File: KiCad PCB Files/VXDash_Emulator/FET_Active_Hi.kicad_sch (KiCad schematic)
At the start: 11 parts, among them J8 Manual backup, Q24 2N7002

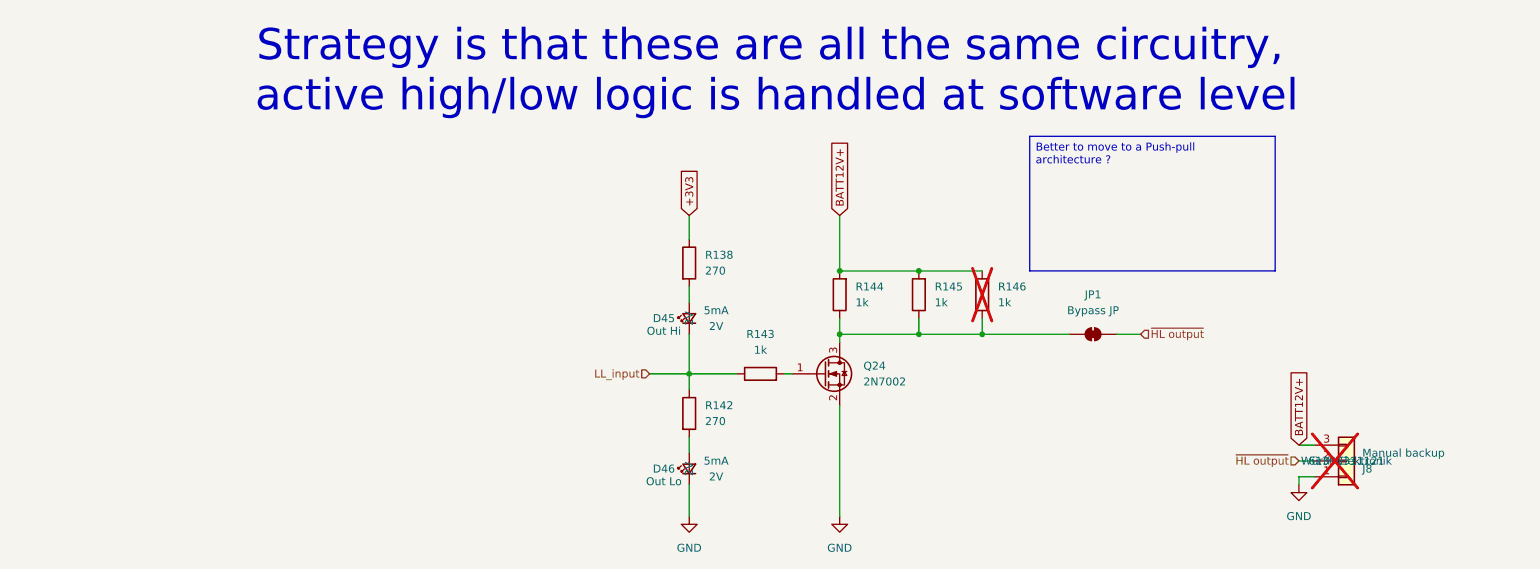
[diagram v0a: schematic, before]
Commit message: Emulator : LCSC part numbers and production files
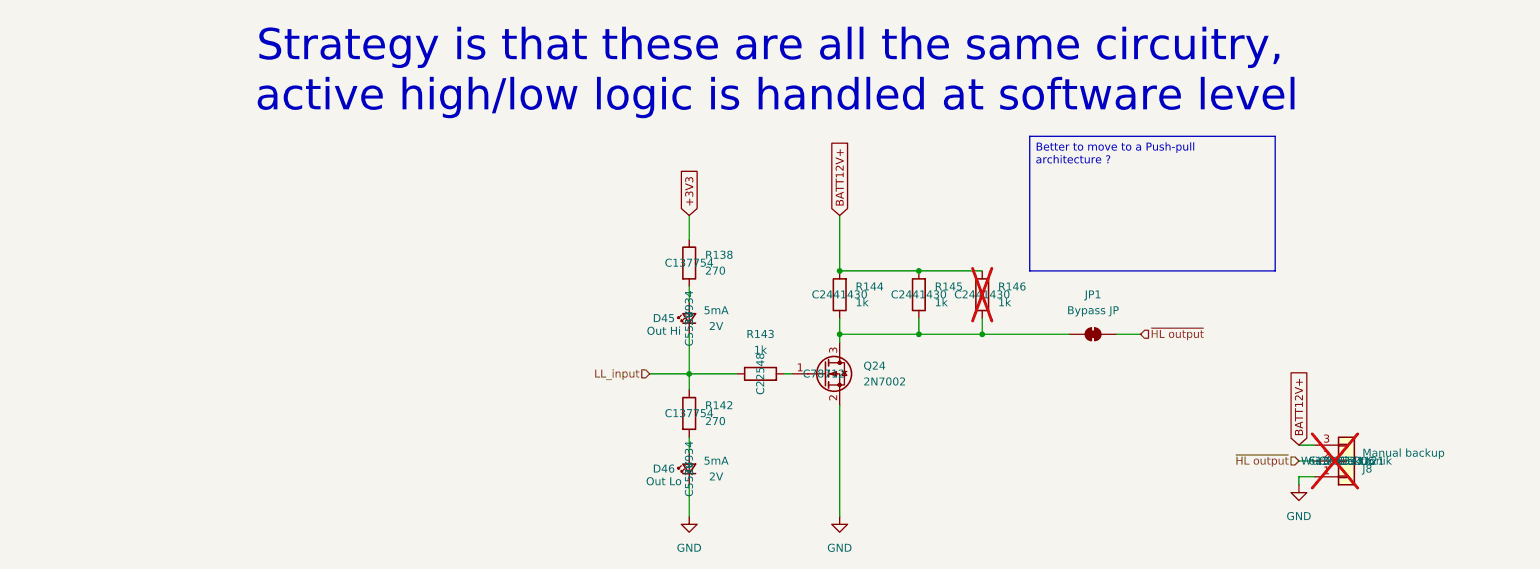
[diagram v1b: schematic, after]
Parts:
- D45, D46: LCSC (none) -> C5556934
- J8: LCSC (none) -> C2915006
- Q24: LCSC (none) -> C78712
- R138, R142: LCSC (none) -> C137754
- R143: LCSC (none) -> C22548
- R144, R145, R146: LCSC (none) -> C2441430
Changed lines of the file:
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@@
+			)
+		)
+		(property "LCSC" "C2915006"
+			(at 201.93 83.82 0)
+			(effects
+				(font
+					(size 1.27 1.27)
+				)
 			)
 		)
@@
 			)
 		)
+		(property "LCSC" "C2441430"
+			(at 120.65 57.15 0)
+			(effects
+				(font
+					(size 1.27 1.27)
+				)
+			)
+		)
 		(pin "1"
 		)
@@
 			)
 		)
+		(property "LCSC" "C78712"
+			(at 118.11 69.85 0)
+			(effects
+				(font
+					(size 1.27 1.27)
+				)
+			)
+		)
 		(pin "1"
 		)
@@
 		)
 		(property "Voltage" "2V"
+			(at 96.52 85.09 0)
+			(effects
+				(font
+					(size 1.27 1.27)
+				)
+			)
+		)
+		(property "LCSC" "C5556934"
 			(at 96.52 85.09 0)
 			(effects
@@
 			)
 		)
+		(property "LCSC" "C137754"
+			(at 96.52 76.2 0)
+			(effects
+				(font
+					(size 1.27 1.27)
+				)
+			)
+		)
 		(pin "1"
 		)
@@
 			)
 		)
+		(property "LCSC" "C22548"
+			(at 107.95 69.85 0)
+			(effects
+				(font
+					(size 1.27 1.27)
+				)
+			)
+		)
 		(pin "1"
 		)
@@
 			)
 		)
+		(property "LCSC" "C137754"
+			(at 96.52 52.07 0)
+			(effects
+				(font
+					(size 1.27 1.27)
+				)
+			)
+		)
 		(pin "1"
 		)
@@
 		)
 		(property "Voltage" "2V"
+			(at 96.52 60.96 0)
+			(effects
+				(font
+					(size 1.27 1.27)
+				)
+			)
+		)
+		(property "LCSC" "C5556934"
 			(at 96.52 60.96 0)
 			(effects
@@
 			)
 		)
+		(property "LCSC" "C2441430"
+			(at 133.35 57.15 0)
+			(effects
+				(font
+					(size 1.27 1.27)
+				)
+			)
+		)
 		(pin "1"
 		)
@@
 			)
 		)
+		(property "LCSC" "C2441430"
+			(at 143.51 57.15 0)
+			(effects
+				(font
+					(size 1.27 1.27)
+				)
+			)
+		)
 		(pin "1"
 		)
@@
 			)
 		)
+		(property "LCSC" ""
+			(at 161.29 63.5 0)
+			(effects
+				(font
+					(size 1.27 1.27)
+				)
+			)
+		)

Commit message: Emulator : Updating BOM with LCSC alts
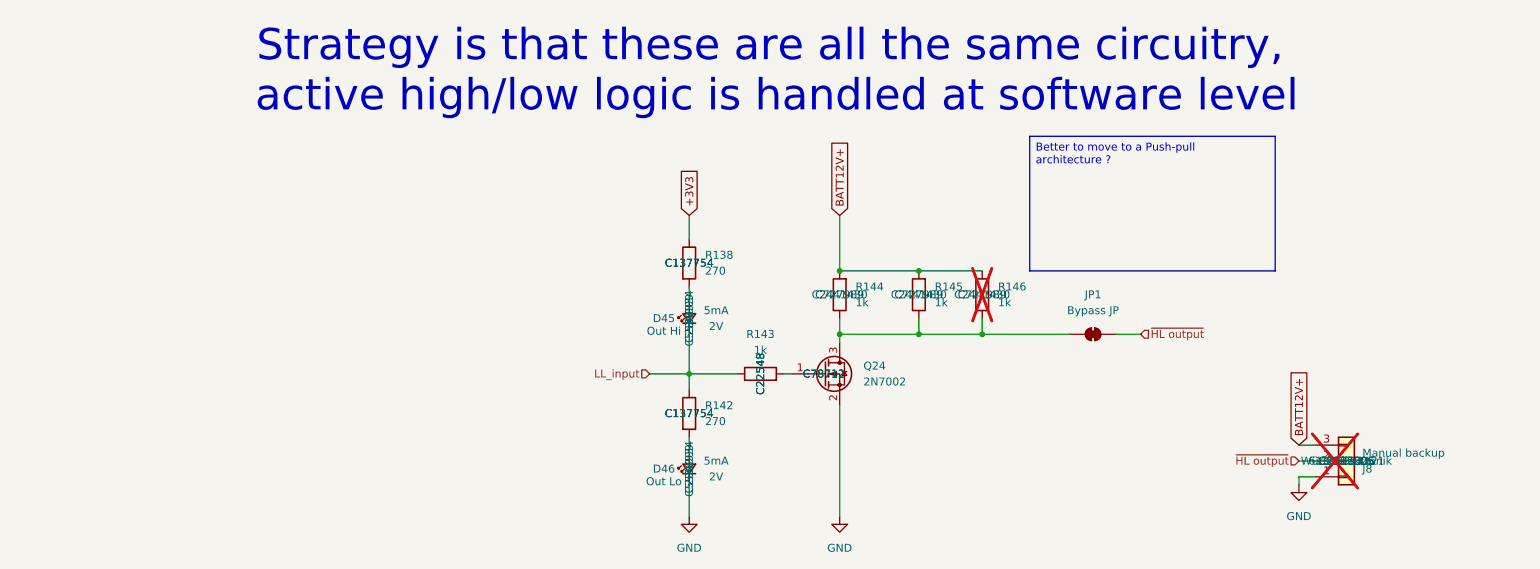
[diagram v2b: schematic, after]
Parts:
- D45, D46: LCSC alt (none) -> C284909
- J8: LCSC alt (none) -> C2937625
- Q24: LCSC alt (none) -> C78712
- R138, R142: LCSC alt (none) -> C137754
- R143: LCSC alt (none) -> C22548
- R144, R145, R146: LCSC alt (none) -> C727989
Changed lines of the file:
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@@
+			)
+		)
+		(property "LCSC alt" "C2937625"
+			(at 201.93 83.82 0)
+			(effects
+				(font
+					(size 1.27 1.27)
+				)
 			)
 		)
@@
 			)
 		)
+		(property "LCSC alt" "C727989"
+			(at 120.65 57.15 0)
+			(effects
+				(font
+					(size 1.27 1.27)
+				)
+			)
+		)
 		(pin "1"
 		)
@@
 			)
 		)
+		(property "LCSC alt" "C78712"
+			(at 118.11 69.85 0)
+			(effects
+				(font
+					(size 1.27 1.27)
+				)
+			)
+		)
 		(pin "1"
 		)
@@
 		)
 		(property "LCSC" "C5556934"
+			(at 96.52 85.09 0)
+			(effects
+				(font
+					(size 1.27 1.27)
+				)
+			)
+		)
+		(property "LCSC alt" "C284909"
 			(at 96.52 85.09 0)
 			(effects
@@
 			)
 		)
+		(property "LCSC alt" "C137754"
+			(at 96.52 76.2 0)
+			(effects
+				(font
+					(size 1.27 1.27)
+				)
+			)
+		)
 		(pin "1"
 		)
@@
 			)
 		)
+		(property "LCSC alt" "C22548"
+			(at 107.95 69.85 0)
+			(effects
+				(font
+					(size 1.27 1.27)
+				)
+			)
+		)
 		(pin "1"
 		)
@@
 			)
 		)
+		(property "LCSC alt" "C137754"
+			(at 96.52 52.07 0)
+			(effects
+				(font
+					(size 1.27 1.27)
+				)
+			)
+		)
 		(pin "1"
 		)
@@
 		)
 		(property "LCSC" "C5556934"
+			(at 96.52 60.96 0)
+			(effects
+				(font
+					(size 1.27 1.27)
+				)
+			)
+		)
+		(property "LCSC alt" "C284909"
 			(at 96.52 60.96 0)
 			(effects
@@
 			)
 		)
+		(property "LCSC alt" "C727989"
+			(at 133.35 57.15 0)
+			(effects
+				(font
+					(size 1.27 1.27)
+				)
+			)
+		)
 		(pin "1"
 		)
@@
 			)
 		)
+		(property "LCSC alt" "C727989"
+			(at 143.51 57.15 0)
+			(effects
+				(font
+					(size 1.27 1.27)
+				)
+			)
+		)
 		(pin "1"
 		)
@@
 			(at 161.29 63.5 0)
 			(effects
+				(font
+					(size 1.27 1.27)
+				)
+			)
+		)
+		(property "LCSC alt" ""
+			(at 161.29 63.5 0)
+			(effects
